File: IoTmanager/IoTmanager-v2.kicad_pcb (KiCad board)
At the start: 2 copper layers, 50 x 70.7 mm, 65 parts, among them J2 Conn_01x12_Pin, J3 Conn_01x12_Pin, J4-flash1 flash, J5 reset, K3 ZC32F-012-HS3-copy, K5 ZC32F-012-HS3-copy, K6 ZC32F-012-HS3-copy, K7 ZC32F-012-HS3-copy, Q1-pnp1 MMBT5401, Q10-pnp1 MMBT5401, Q11-npn1 MMBT5551-npn, Q5 MMBT5401, Q6 MMBT5551-npn, Q7-npn1 MMBT5551-npn, Q8-pnp1 MMBT5401, Q9 MMBT5551-npn, U12 AMS1117-5.0, U2 ESP-12F, U3-tsop23 TSOP23xx, U4 Mini360, U5 PJ-320A, U6 AMS1117-3.3, U7 DS18B20

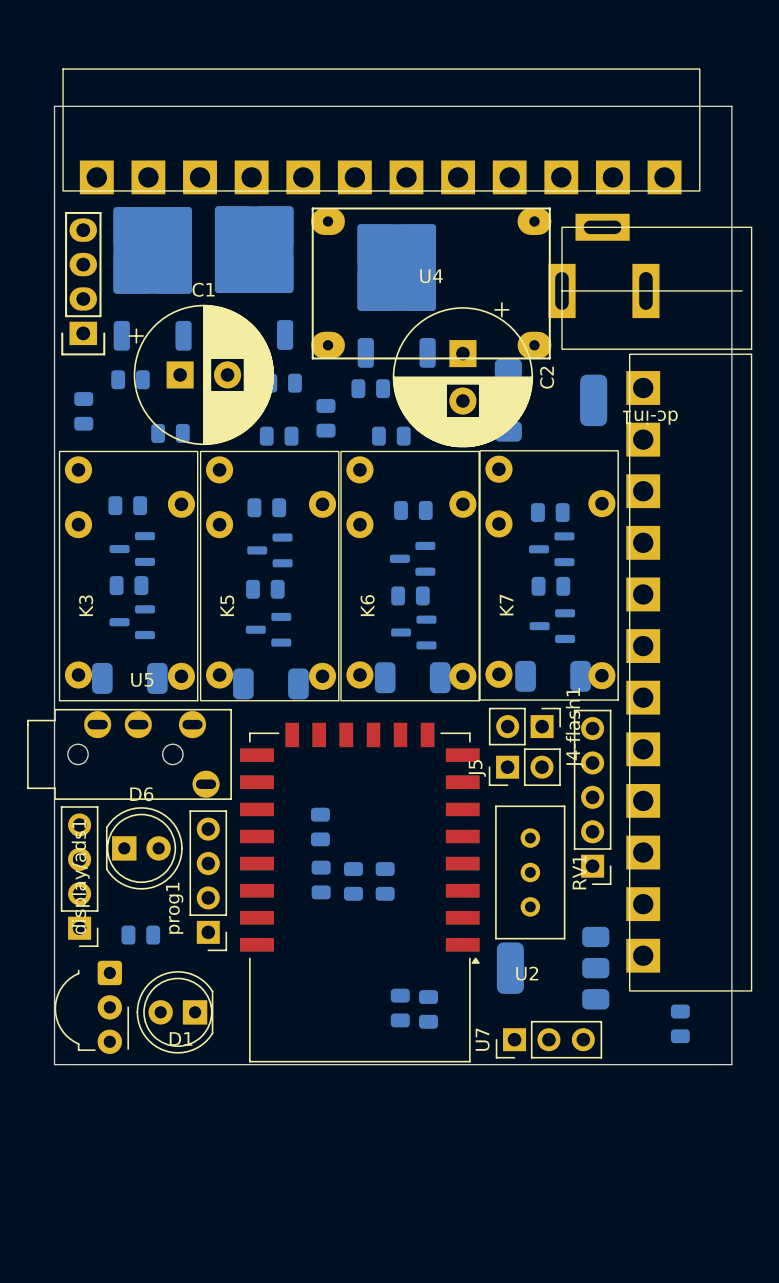
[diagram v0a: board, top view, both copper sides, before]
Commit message: update
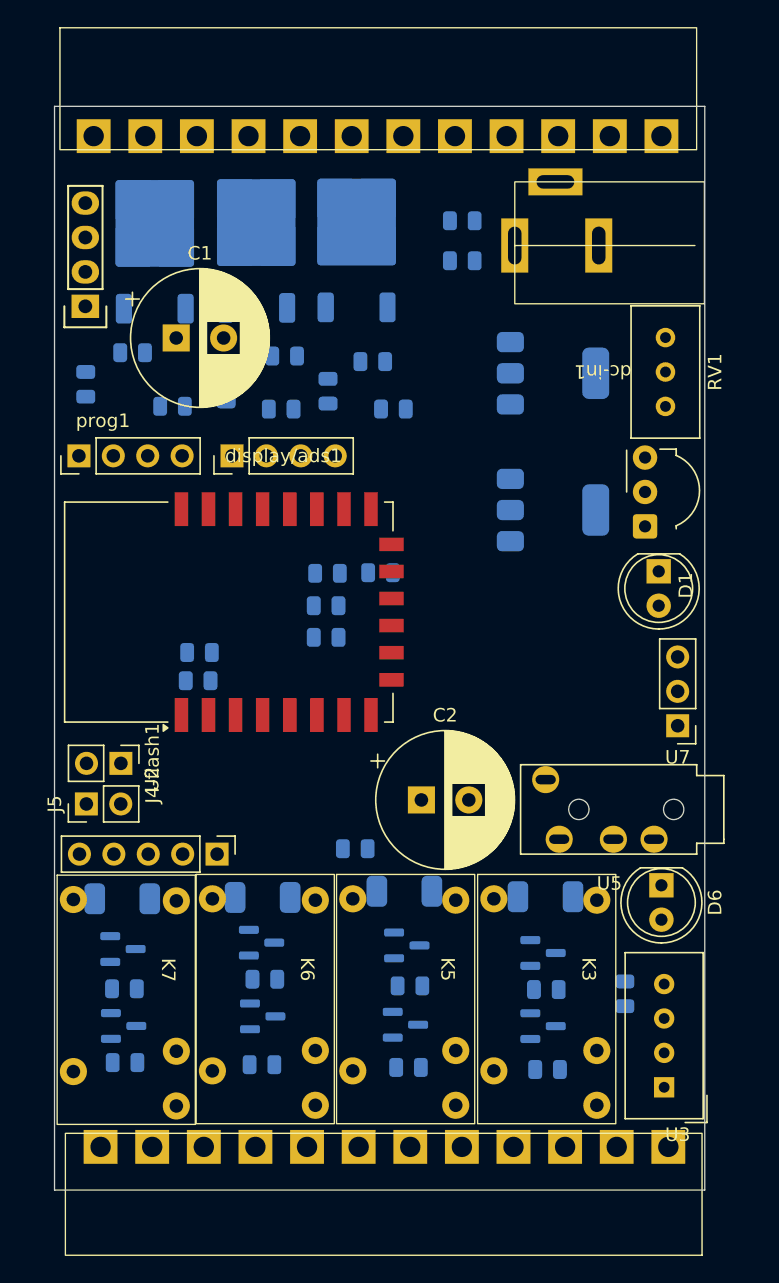
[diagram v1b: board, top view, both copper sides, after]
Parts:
- removed U4: Mini360, module-custom-for-esp8266:Mini360_step-down
- added R12-10k2: R-1k, Resistor_SMD:R_0805_2012Metric, B.Cu at (107.7, 63.4)
- added R12-10k3: R-1k, Resistor_SMD:R_0805_2012Metric, B.Cu at (107.7, 66.3)
- added U3: DHT11, Sensor:Aosong_DHT11_5.5x12.0_P2.54mm, F.Cu at (122.6, 127.3)
- moved U5 52.1 mm to (127.0, 109.0), turned to 180 degrees
- moved R21 51.9 mm to (114.0, 126.0), turned to 0 degrees
- moved U3-tsop23 51.5 mm to (121.2, 85.9), turned to 90 degrees
- moved R25 51.3 mm to (82.8, 125.5), turned to 180 degrees
- moved Q10-pnp1 47.3 mm to (82.7, 122.8), turned to 0 degrees
- moved D1 47.2 mm to (122.2, 89.2), turned to -90 degrees
- moved Q5 46.5 mm to (113.7, 122.8), turned to 0 degrees
- moved R26 43.3 mm to (82.8, 120.0), turned to 180 degrees
- moved K3 43.0 mm to (119.0, 111.6), turned to -90 degrees
- moved R22 42.9 mm to (113.9, 120.1), turned to 0 degrees
- moved R4 42.6 mm to (103.7, 125.8), turned to 0 degrees
- moved R23 42.4 mm to (92.9, 125.6), turned to 0 degrees
- moved J2 41.8 mm to (80.0, 130.7), turned to 180 degrees
- moved D6 39.7 mm to (122.4, 112.4), turned to -90 degrees
- moved Q11-npn1 39.7 mm to (82.7, 117.1), turned to 0 degrees
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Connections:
- J2 pad 9: /d0 -> unconnected-(J2-Pin_9-Pad9)
- Jumper-d5 pad 1: /d5 -> Net-(IRLR2-G)
- Jumper-d6 pad 1: /d6 -> Net-(IRLR1-G)
- Jumper-d7 pad 1: /d7 -> Net-(IRLR3-G)
- U2 pad 19: /d2 -> Net-(U2-GPIO4)
- U2 pad 20: /d1 -> Net-(U2-GPIO5)
- U3-tsop23 pad 1: /d5 -> /d1
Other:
- board size 50 x 70.7 mm -> 48 x 80 mm
